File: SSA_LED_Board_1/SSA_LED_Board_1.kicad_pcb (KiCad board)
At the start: 2 copper layers, 75 x 50 mm, 0 parts

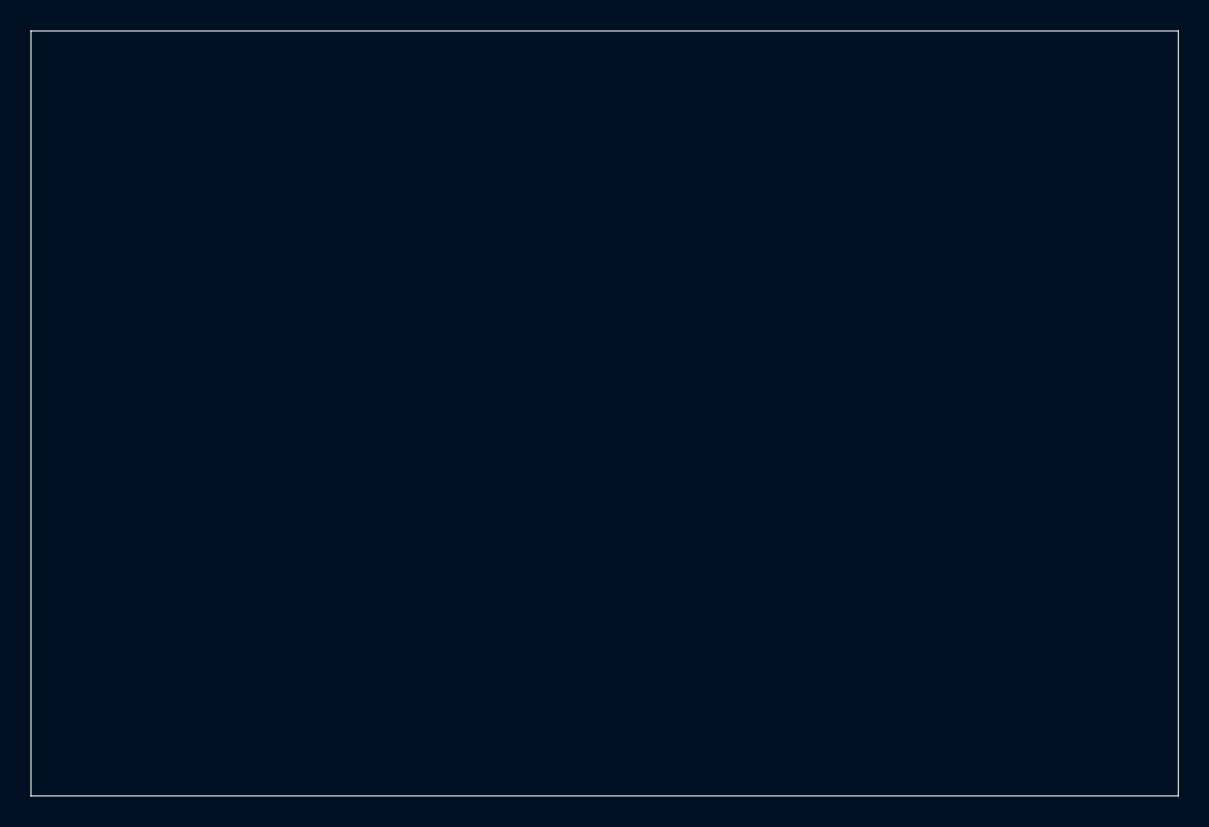
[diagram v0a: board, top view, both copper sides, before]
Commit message: finished layout
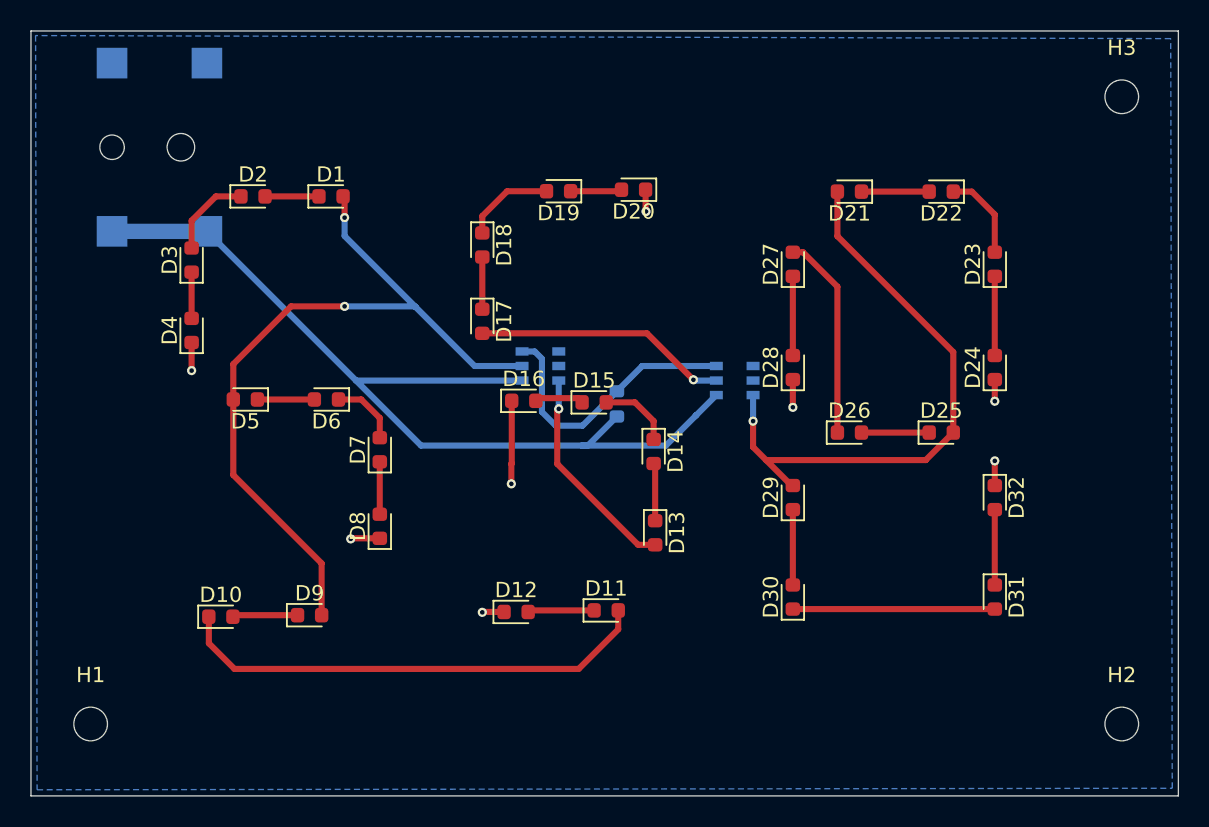
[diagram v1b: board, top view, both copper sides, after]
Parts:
- added D1: D, Diode_SMD:D_0603_1608Metric, F.Cu at (39.6, 30.8)
- added D10: D, Diode_SMD:D_0603_1608Metric, F.Cu at (32.4, 58.3)
- added D11: D, Diode_SMD:D_0603_1608Metric, F.Cu at (57.6, 57.9)
- added D12: D, Diode_SMD:D_0603_1608Metric, F.Cu at (51.7, 58.0)
- added D13: D, Diode_SMD:D_0603_1608Metric, F.Cu at (60.8, 52.8)
- added D14: D, Diode_SMD:D_0603_1608Metric, F.Cu at (60.7, 47.5)
- added D15: D, Diode_SMD:D_0603_1608Metric, F.Cu at (56.8, 44.3)
- added D16: D, Diode_SMD:D_0603_1608Metric, F.Cu at (52.2, 44.2)
- added D17: D, Diode_SMD:D_0603_1608Metric, F.Cu at (49.5, 39.0)
- added D18: D, Diode_SMD:D_0603_1608Metric, F.Cu at (49.5, 34.0)
- added D19: D, Diode_SMD:D_0603_1608Metric, F.Cu at (54.5, 30.5)
- added D2: D, Diode_SMD:D_0603_1608Metric, F.Cu at (34.5, 30.8)
- added D20: D, Diode_SMD:D_0603_1608Metric, F.Cu at (59.4, 30.4)
- added D21: D, Diode_SMD:D_0603_1608Metric, F.Cu at (73.5, 30.5)
- added D22: D, Diode_SMD:D_0603_1608Metric, F.Cu at (79.5, 30.5)
- added D23: D, Diode_SMD:D_0603_1608Metric, F.Cu at (83.0, 35.2)
- added D24: D, Diode_SMD:D_0603_1608Metric, F.Cu at (83.0, 42.0)
- added D25: D, Diode_SMD:D_0603_1608Metric, F.Cu at (79.5, 46.2)
- added D26: D, Diode_SMD:D_0603_1608Metric, F.Cu at (73.5, 46.2)
- added D27: D, Diode_SMD:D_0603_1608Metric, F.Cu at (69.8, 35.2)
- added D28: D, Diode_SMD:D_0603_1608Metric, F.Cu at (69.8, 42.0)
- added D29: D, Diode_SMD:D_0603_1608Metric, F.Cu at (69.8, 50.5)
- added D3: D, Diode_SMD:D_0603_1608Metric, F.Cu at (30.5, 35.0)
- added D30: D, Diode_SMD:D_0603_1608Metric, F.Cu at (69.8, 57.0)
- added D31: D, Diode_SMD:D_0603_1608Metric, F.Cu at (83.0, 57.0)
- added D32: D, Diode_SMD:D_0603_1608Metric, F.Cu at (83.0, 50.5)
- added D4: D, Diode_SMD:D_0603_1608Metric, F.Cu at (30.5, 39.6)
- added D5: D, Diode_SMD:D_0603_1608Metric, F.Cu at (34.0, 44.1)
- added D6: D, Diode_SMD:D_0603_1608Metric, F.Cu at (39.3, 44.1)
- added D7: D, Diode_SMD:D_0603_1608Metric, F.Cu at (42.8, 47.4)
- added D8: D, Diode_SMD:D_0603_1608Metric, F.Cu at (42.8, 52.4)
- added D9: D, Diode_SMD:D_0603_1608Metric, F.Cu at (38.2, 58.2)
- added H1: MountingHole, MountingHole:MountingHole_2.2mm_M2, F.Cu at (23.9, 65.3)
- added H2: MountingHole, MountingHole:MountingHole_2.2mm_M2, F.Cu at (91.3, 65.3)
- added H3: MountingHole, MountingHole:MountingHole_2.2mm_M2, F.Cu at (91.3, 24.3)
- added J1: 54-00164, 54-00164:TENSILITY_54-00164, B.Cu at (27.6, 27.6)
- added R1: 25 ohms, Resistor_SMD:R_0603_1608Metric, B.Cu at (58.3, 44.4)
- added U1: BCR401U, BCR401U:SOP95P250X110-6N-1, B.Cu at (53.3, 41.9)
- added U2: BCR401U, BCR401U:SOP95P250X110-6N-1, B.Cu at (66.0, 42.9)
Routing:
- net /D_string_1: track 0.00 -> 64.1 mm, vias 0 -> 3
- net /Power_in: track 0.00 -> 60.7 mm
- net /D_string_5: track 0.00 -> 55.5 mm, vias 0 -> 2
- net Net-(D10-K): track 0.00 -> 31.5 mm
- net /REXT: track 0.00 -> 18.4 mm
- net GND: track 0.00 -> 16.9 mm, vias 0 -> 8
- net Net-(D26-K): track 0.00 -> 13.4 mm
- net Net-(D30-K): track 0.00 -> 13.2 mm
- net Net-(D18-K): track 0.00 -> 5.97 mm
- net Net-(D22-K): track 0.00 -> 5.80 mm
- net Net-(D2-K): track 0.00 -> 5.67 mm
- net Net-(D27-K): track 0.00 -> 5.17 mm
- net Net-(D23-K): track 0.00 -> 5.17 mm
- net Net-(D31-K): track 0.00 -> 4.92 mm
- net Net-(D29-K): track 0.00 -> 4.92 mm
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- added copper zone on B.Cu, net GND
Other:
- board text added: "Designed By: Matthew Scala"
